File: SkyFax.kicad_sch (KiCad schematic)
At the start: 59 parts, among them J1 RJ11/12, J2 DE9_Receptacle_MountingHoles, J3 Conn_01x02, Q1 Q_NPN_BEC, Q2 Q_PNP_BEC, Q3 Q_NPN_BEC, Q4 Q_NPN_BEC, Q5 Q_NPN_BEC, Q6 Q_NPN_EBC, SW1 SW_DIP_x08, SW2 SW_Push, U1 Si2494-A-FM, U2 Si3018, U3 25LC640AT-E/SN, X1 ECS-2520MV-xxx-xx

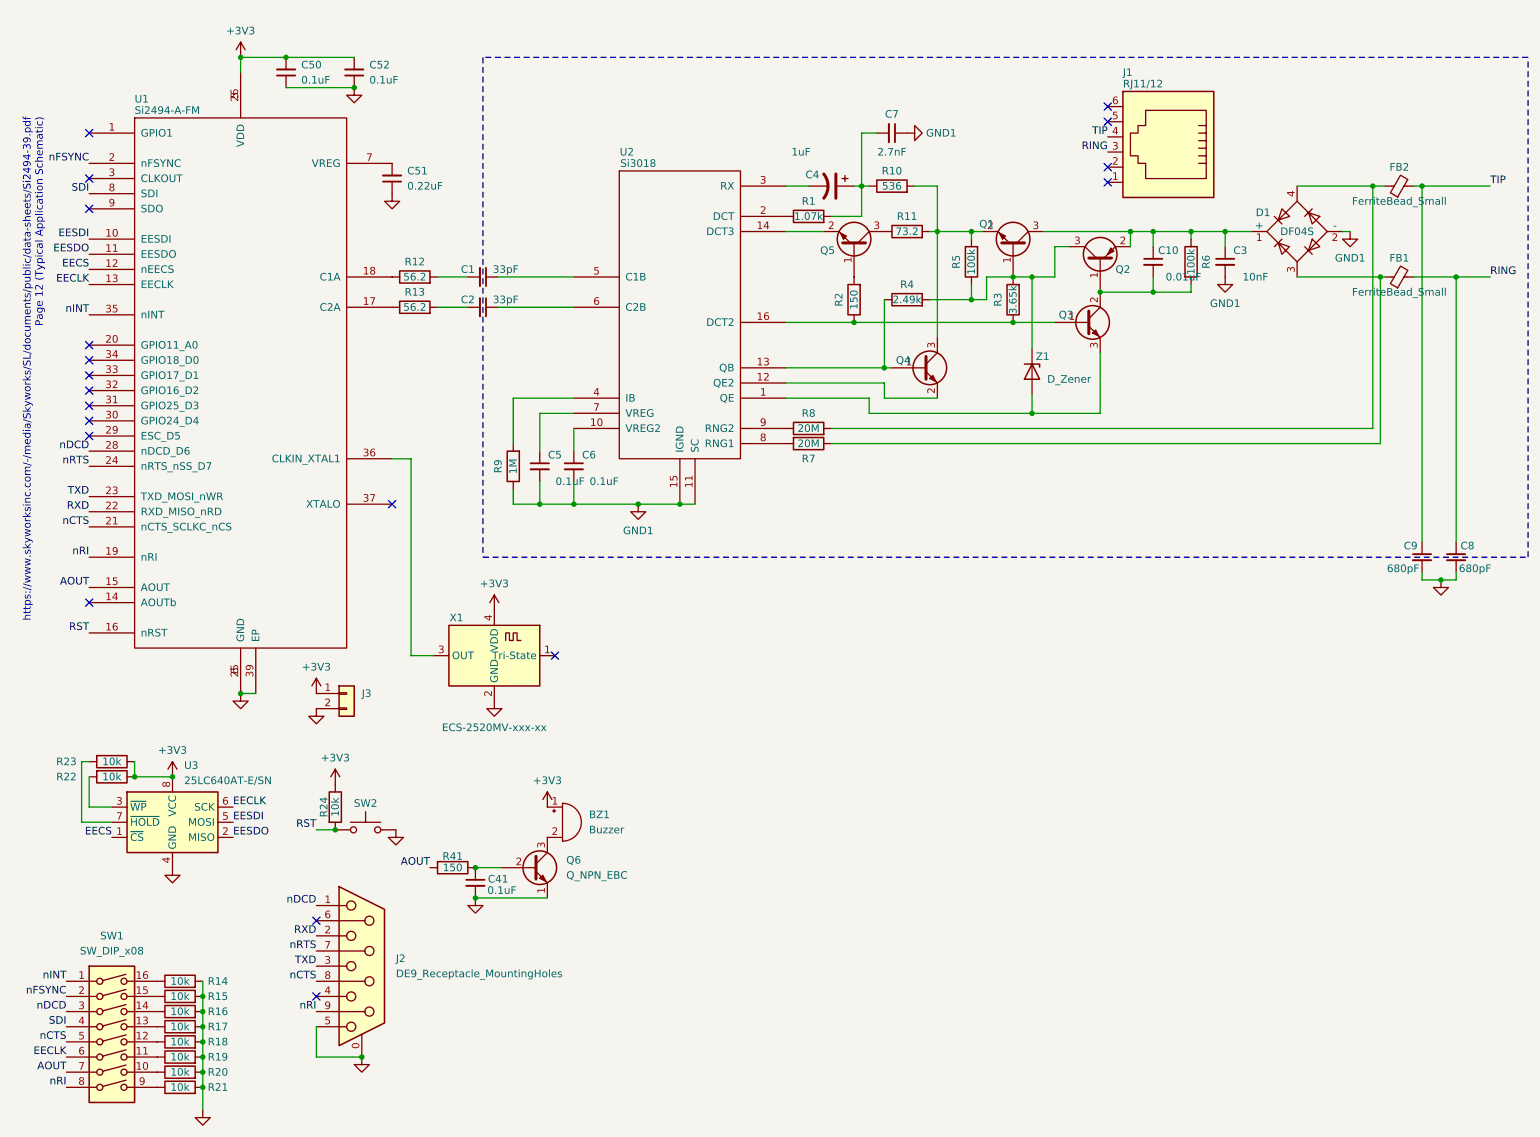
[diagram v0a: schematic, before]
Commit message: Version 2.0 Schematics
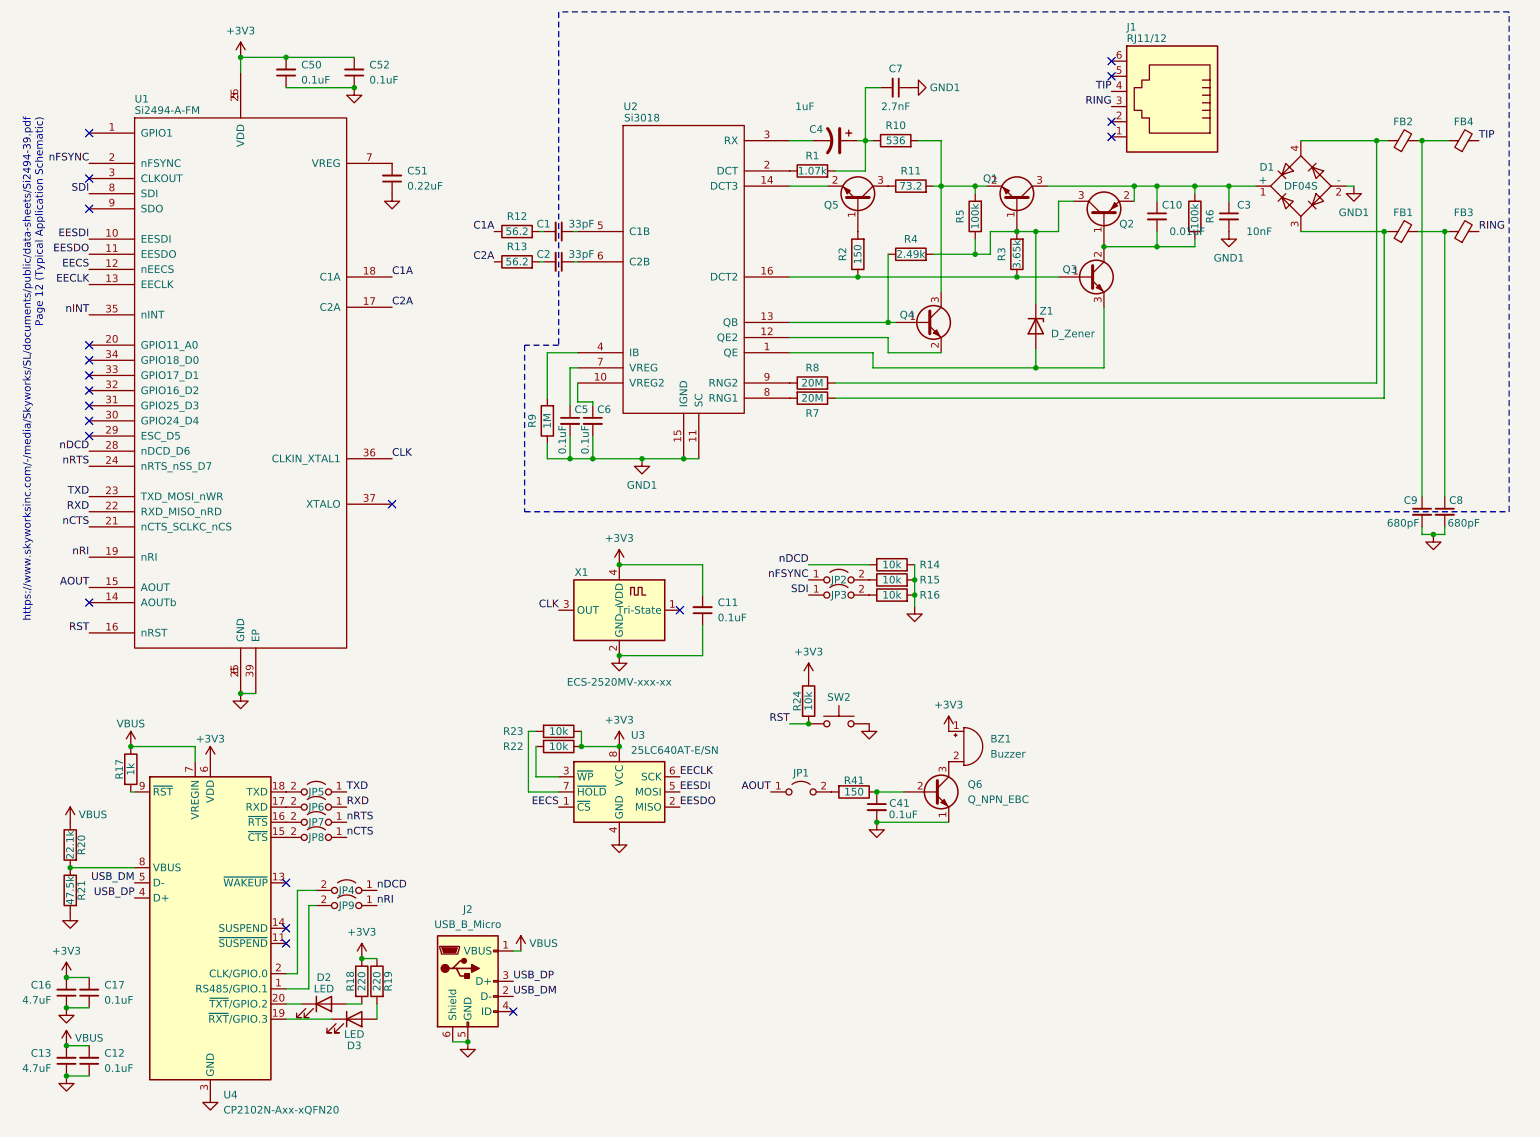
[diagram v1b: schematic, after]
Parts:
- removed J2: DE9_Receptacle_MountingHoles, Connector_Dsub:DSUB-9_Female_Horizontal_P2.77x2.84mm_EdgePinOffset9.90mm_Housed_MountingHolesOffset11.32mm, symbol Connector:DE9_Receptacle_MountingHoles
- removed J3: Conn_01x02, Connector_PinHeader_2.54mm:PinHeader_1x02_P2.54mm_Vertical, symbol Connector_Generic:Conn_01x02
- removed SW1: SW_DIP_x08, Button_Switch_SMD:SW_DIP_SPSTx08_Slide_6.7x21.88mm_W6.73mm_P2.54mm_LowProfile_JPin, symbol Switch:SW_DIP_x08
- added C11, C12, C17: 0.1uF, Capacitor_SMD:C_0603_1608Metric, symbol Device:C_Small
- added C13, C16: 4.7uF, Capacitor_SMD:C_0402_1005Metric, symbol Device:C_Small
- added D2, D3: LED, LED_SMD:LED_0201_0603Metric, symbol Device:LED
- added FB3, FB4: FerriteBead_Small, Inductor_SMD:L_0805_2012Metric, symbol Device:FerriteBead_Small
- added J2: USB_B_Micro, Connector_USB:USB_Micro-B_Amphenol_10118193-0001LF_Horizontal, symbol Connector:USB_B_Micro
- added JP1, JP2, JP3, JP4, JP5, JP6, JP7, JP8, JP9: Jumper_2_Open, Connector_PinHeader_2.54mm:PinHeader_1x02_P2.54mm_Vertical, symbol Jumper:Jumper_2_Open
- added U4: CP2102N-Axx-xQFN20, Package_DFN_QFN:SiliconLabs_QFN-20-1EP_3x3mm_P0.5mm, symbol Interface_USB:CP2102N-Axx-xQFN20
- R17: value 10k -> 1k; footprint Resistor_SMD:R_0603_1608Metric -> Resistor_SMD:R_0402_1005Metric; DIGIKEY RNCP0603FTD10K0CT-ND -> 311-1.0KJRCT-ND
- R18, R19: value 10k -> 220; footprint Resistor_SMD:R_0603_1608Metric -> Resistor_SMD:R_0402_1005Metric; DIGIKEY RNCP0603FTD10K0CT-ND -> 1292-WR04X2200FTLCT-ND
- R20: value 10k -> 22.1k; footprint Resistor_SMD:R_0603_1608Metric -> Resistor_SMD:R_0402_1005Metric; DIGIKEY RNCP0603FTD10K0CT-ND -> 311-22.1KLRCT-ND
- R21: value 10k -> 47.5k; footprint Resistor_SMD:R_0603_1608Metric -> Resistor_SMD:R_0402_1005Metric; DIGIKEY RNCP0603FTD10K0CT-ND -> 311-47.5KLRCT-ND
- SW2: footprint (none) -> Button_Switch_SMD:SW_Tactile_SPST_NO_Straight_CK_PTS636Sx25SMTRLFS; DIGIKEY (none) -> CKN12322-1-ND
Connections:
- net +3V3: now also R18.1, R19.1, C11.2, C16.2, C17.2, U4.6 (VDD)
- net AOUT: now also JP1.1 (A); no longer R41.2
- net GND: now also C11.1, C12.1, C13.1, C16.1, C17.1, J2.5 (GND), J2.6 (Shield), U4.12 (GND), U4.21 (GND), U4.3 (GND); no longer R17.2, R18.2, R19.2, R20.2
- net RING: now also FB3.2; no longer C8.1, FB1.2
- net RXD: now also JP6.1 (A)
- net SDI: now also JP3.1 (A)
- net TIP: now also FB4.2; no longer C9.1, FB2.2
- net TXD: now also JP5.1 (A)
- net nCTS: now also JP8.1 (A)
- net nDCD: now also R14.1, JP4.1 (A)
- net nFSYNC: now also JP2.1 (A)
- net nRI: now also JP9.1 (A)
- net nRTS: now also JP7.1 (A)
- net C2A: now reaches R13.1, U1.17 (C2A)
- net VBUS: now reaches R17.1
- net VBUS: now also R20.1, C12.2, C13.2, J2.1 (VBUS), U4.7 (VREGIN)
- net C1A: now reaches R12.1, U1.18 (C1A)
- net CLK: now reaches U1.36 (CLKIN_XTAL1), X1.3 (OUT)
- net at R21.1: now also R20.2, U4.8 (VBUS)
- net at R15.1: now also JP2.2 (B)
- net at R16.1: now also JP3.2 (B)
- new net: C9.1, FB2.2, FB4.1
- new net: D2.2 (A), R18.2
- new net: JP9.2 (B), U4.1 (RS485/GPIO.1)
- new net: JP7.2 (B), U4.16 (~{RTS})
- new net: D3.2 (A), R19.2
- new net: D3.1 (K), U4.19 (~{RXT}/GPIO.3)
- new net: JP1.2 (B), R41.2
- new net: JP5.2 (B), U4.18 (TXD)
- new net: D2.1 (K), U4.20 (~{TXT}/GPIO.2)
- new net: JP8.2 (B), U4.15 (~{CTS})
- new net: JP6.2 (B), U4.17 (RXD)
- new net: JP4.2 (B), U4.2 (CLK/GPIO.0)
- new net: R17.2, U4.9 (~{RST})
- new net: C8.1, FB1.2, FB3.1
- new net USB_DM: J2.2 (D-), U4.5 (D-)
- new net USB_DP: J2.3 (D+), U4.4 (D+)
- no-connect marks 19 -> 21
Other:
- moved on the sheet: BZ1, C1, C10, C2, C3, C4, C41, C5, C6, C7, C8, C9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
